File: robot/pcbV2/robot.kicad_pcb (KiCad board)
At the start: 2 copper layers, 70 x 100 mm, 29 parts, among them J1 Conn_01x02_Female, J2 Conn_01x06_Male, J3 Conn_01x06_Male, J4 Conn_01x05_Female, J5 Conn_01x05_Female, U1 ESP32_NODEMCU, U2 L7812, U3 L7805

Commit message: dopisany tekst w latexie
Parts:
- moved C10 45.5 mm to (101.7, 131.0)
- moved C11 45.5 mm to (125.7, 124.0)
- moved C2 45.5 mm to (104.7, 140.0)
- moved C3 45.5 mm to (134.7, 123.0)
- moved C4 45.5 mm to (86.7, 57.0)
- moved C7 45.5 mm to (89.7, 123.0)
- moved C8 45.5 mm to (89.7, 129.0)
- moved C9 45.5 mm to (95.7, 142.5)
- moved D1 45.5 mm to (123.7, 138.0)
- moved D11 45.5 mm to (142.3, 111.0)
- moved D12 45.5 mm to (142.3, 100.0)
- moved D13 45.5 mm to (142.3, 89.0)
- moved D2 45.5 mm to (123.7, 131.0)
- moved D3 45.5 mm to (98.7, 138.5)
- moved F1 45.5 mm to (139.7, 132.0)
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
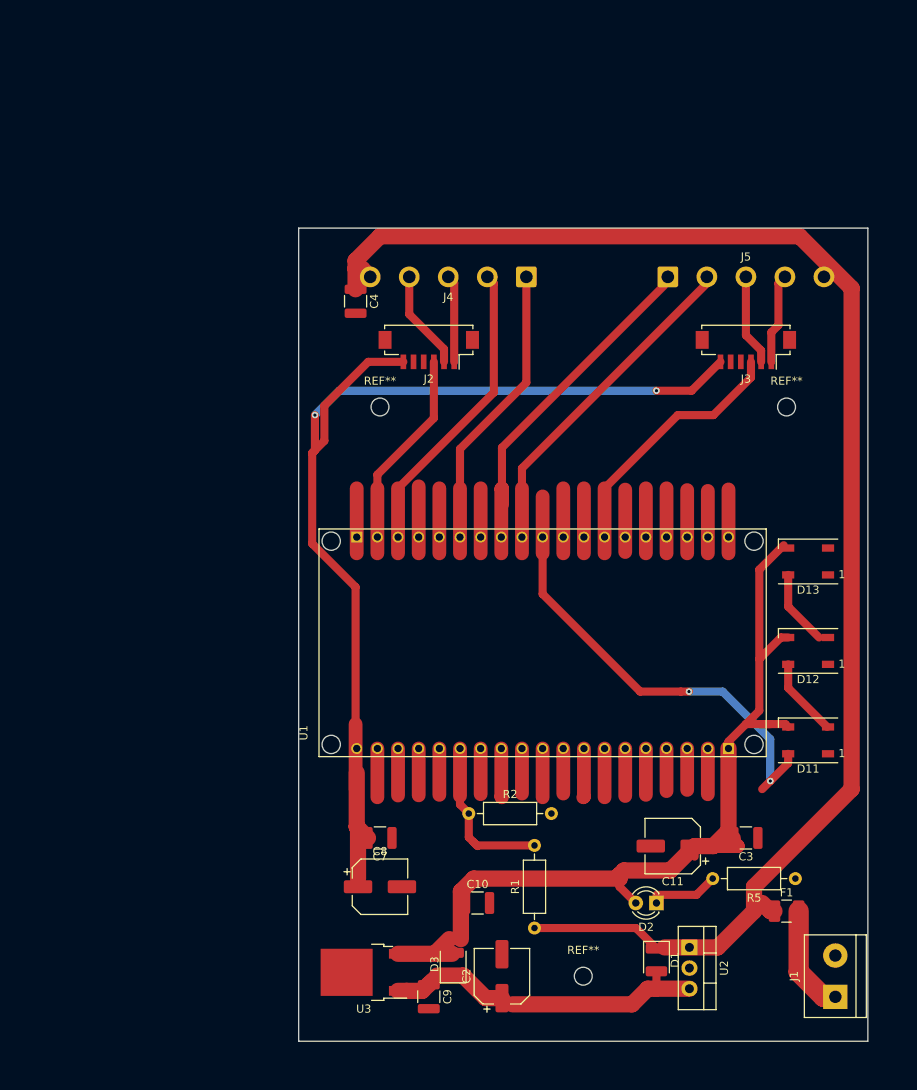
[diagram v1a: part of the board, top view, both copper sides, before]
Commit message: robot
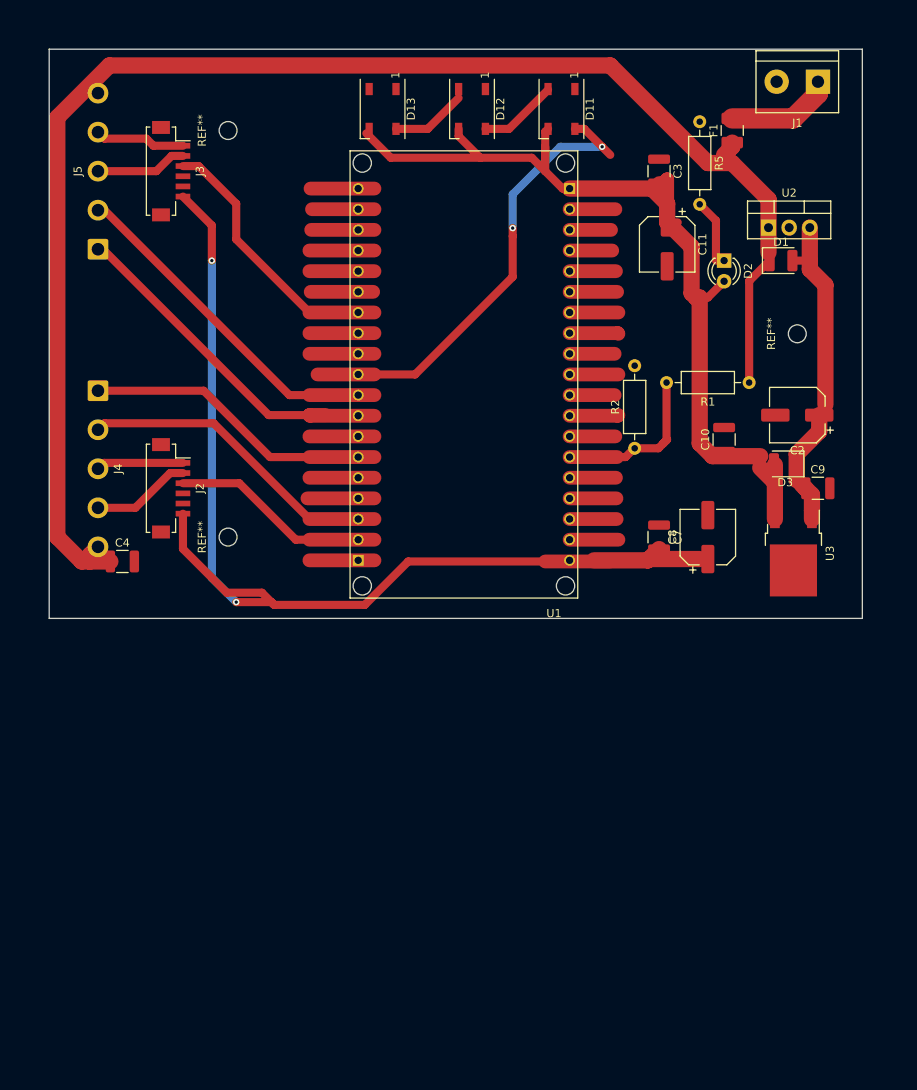
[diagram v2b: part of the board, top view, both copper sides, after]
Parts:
- moved J1 112.6 mm to (143.5, 30.0), turned to 180 degrees
- moved F1 96.2 mm to (133.0, 36.0), turned to 90 degrees
- moved R5 93.8 mm to (129.0, 34.9), turned to -90 degrees
- moved U2 89.0 mm to (137.5, 47.9), turned to 0 degrees
- moved D1 87.4 mm to (139.0, 52.0), turned to 0 degrees
- moved D11 83.4 mm to (112.0, 33.4), turned to -90 degrees
- moved REF** 83.3 mm to (141.0, 61.0), turned to 90 degrees
- moved C3 82.7 mm to (124.0, 41.0), turned to -90 degrees
- moved D2 79.4 mm to (132.0, 52.0), turned to -90 degrees
- moved C9 78.7 mm to (143.5, 80.0), turned to 0 degrees
- moved D12 78.4 mm to (101.0, 33.4), turned to -90 degrees
- moved C2 78.0 mm to (141.0, 71.0), turned to 180 degrees
- moved REF** 76.6 mm to (71.0, 36.0), turned to 90 degrees
- moved D13 76.4 mm to (90.0, 33.4), turned to -90 degrees
- moved J3 74.0 mm to (64.0, 41.0), turned to -90 degrees
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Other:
- board size 70 x 100 mm -> 100 x 70 mm
